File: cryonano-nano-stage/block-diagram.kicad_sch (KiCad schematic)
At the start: 10 parts, among them J1 24VDC IN, J2 JST-B2B-XH-AM, J3 JST-B2B-XH-AM, J5 JST-B3B-XH-AM

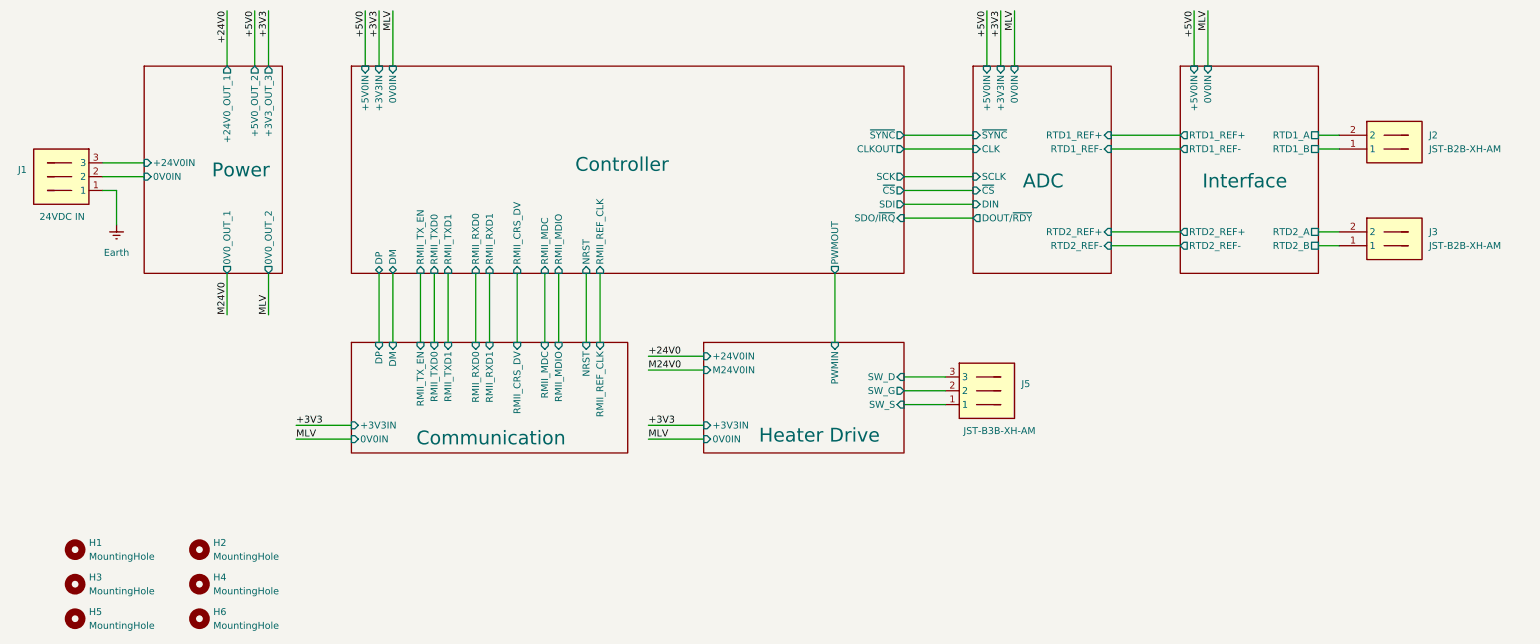
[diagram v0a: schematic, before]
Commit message: sch improved
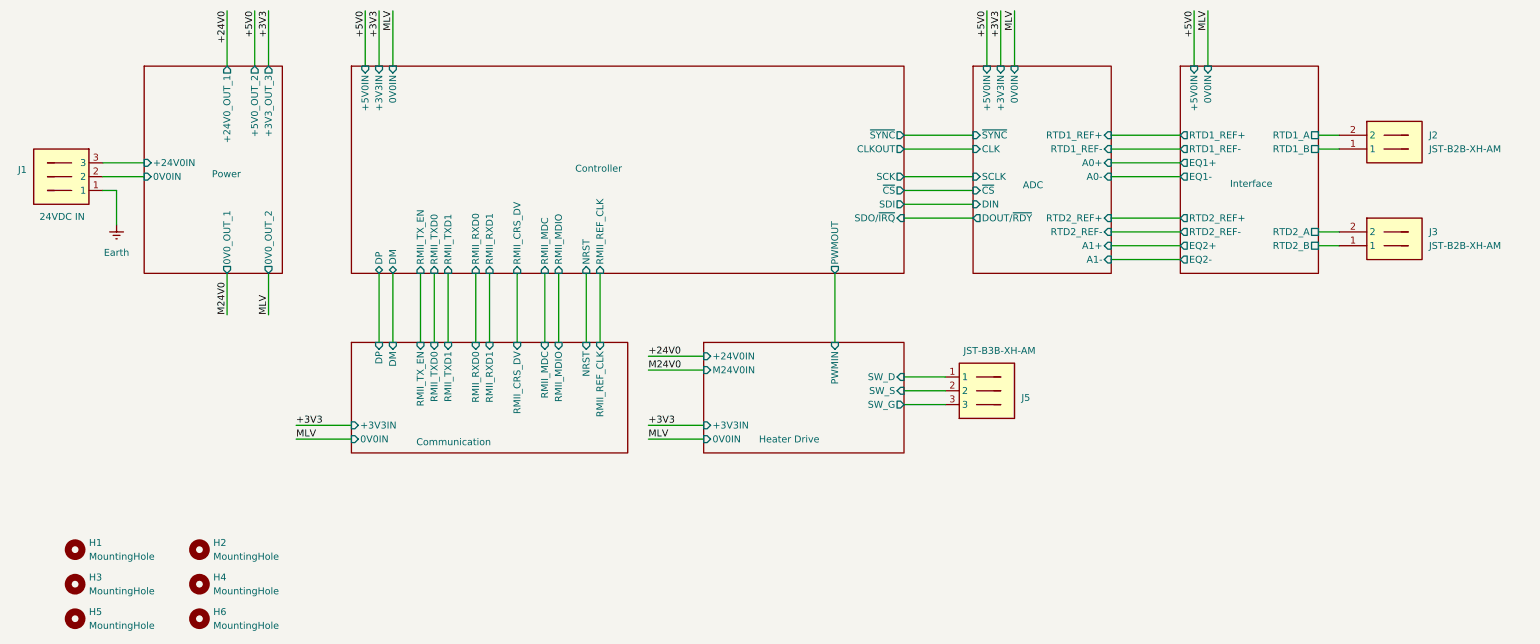
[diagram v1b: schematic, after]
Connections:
- net Heater Drive/SW_D: now also J5.1; no longer J5.3
- net Heater Drive/SW_G: now also J5.3; no longer J5.2
- net Heater Drive/SW_S: now also J5.2; no longer J5.1
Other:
- sheet ADC ports: added A0+, A0-, A1+, A1-; removed none
- sheet Interface ports: added EQ1+, EQ1-, EQ2+, EQ2-; removed none
